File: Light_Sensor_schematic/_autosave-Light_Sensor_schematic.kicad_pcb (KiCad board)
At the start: 2 copper layers, 50 x 50 mm, 21 parts, among them IC1 TSL237S-LF, J1 Conn_01x03, J3 Conn_01x04_Male, U1 STM32L432KCUx, U2 STDC14, U3 TG-3541CE

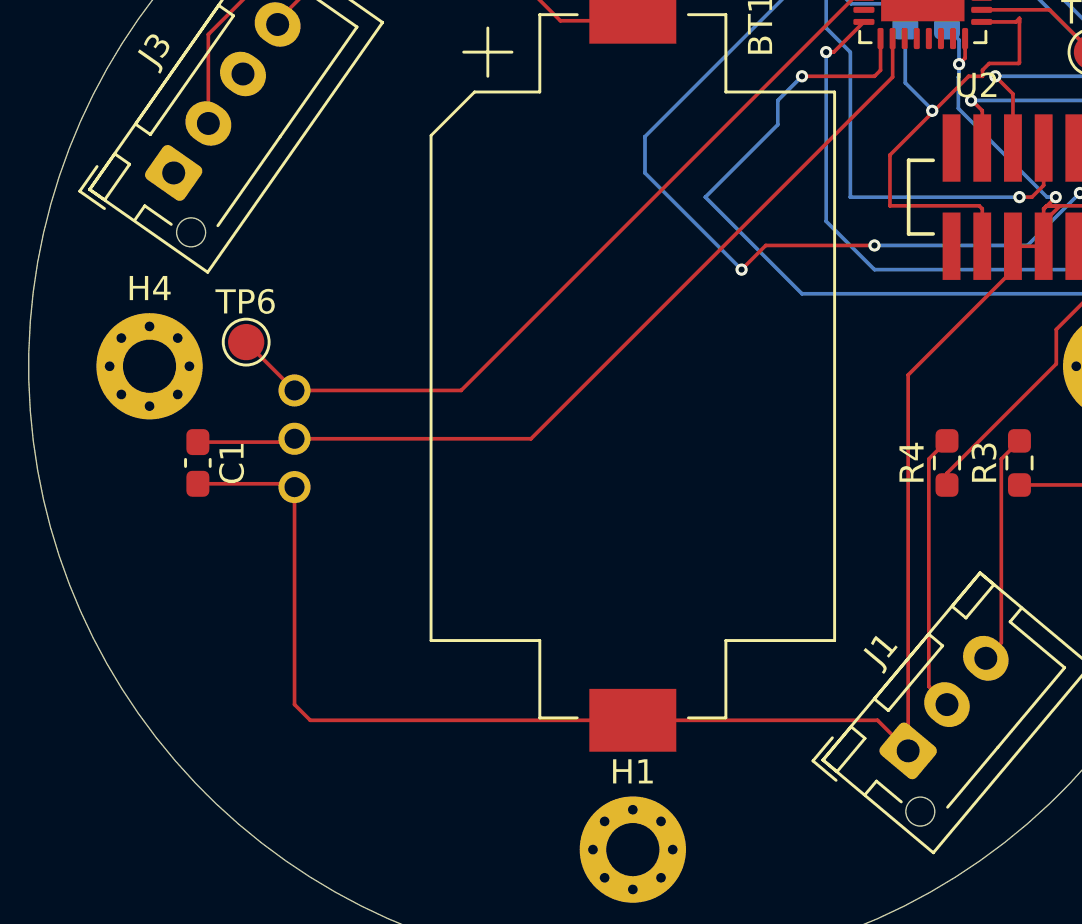
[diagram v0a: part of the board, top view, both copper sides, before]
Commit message: Lab 8
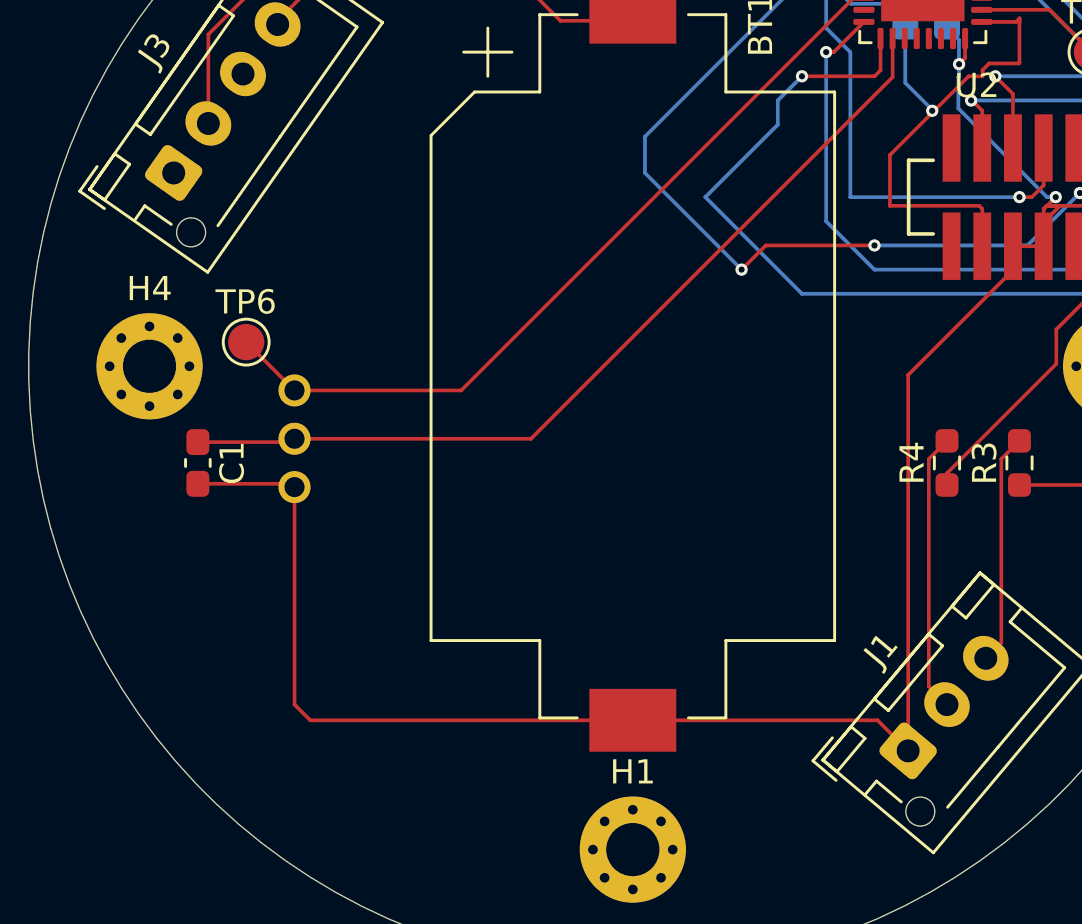
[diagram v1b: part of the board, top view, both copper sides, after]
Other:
- rule pad_to_mask_clearance: 0 -> 0.0508
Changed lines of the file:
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@@
     (pad_size 1.524 1.524)
     (pad_drill 0.762)
-    (pad_to_mask_clearance 0)
+    (pad_to_mask_clearance 0.0508)
     (aux_axis_origin 0 0)
     (visible_elements FFFFFF7F)
@@
       (outputformat 1)
       (mirror false)
-      (drillshape 1)
+      (drillshape 0)
       (scaleselection 1)
       (outputdirectory ""))
@@
       (effects (font (size 1 1) (thickness 0.15)))
     )
-    (pad 1 thru_hole roundrect (at 0 0 50) (size 1.7 1.95) (drill 0.95) (layers *.Cu *.Mask) (roundrect_rratio 0.147059)
+    (pad 1 thru_hole roundrect (at 0 0 50) (size 1.7 1.95) (drill 0.95) (layers *.Cu *.Mask) (roundrect_rratio 0.1470588235294118)
       (net 1 GND))
     (pad 2 thru_hole oval (at 2.5 0 50) (size 1.7 1.95) (drill 0.95) (layers *.Cu *.Mask)
@@
       (effects (font (size 1 1) (thickness 0.15)))
     )
-    (pad 1 thru_hole roundrect (at 0 0 55) (size 1.7 1.95) (drill 0.95) (layers *.Cu *.Mask) (roundrect_rratio 0.147059)
+    (pad 1 thru_hole roundrect (at 0 0 55) (size 1.7 1.95) (drill 0.95) (layers *.Cu *.Mask) (roundrect_rratio 0.1470588235294118)
       (net 8 "Net-(J3-Pad1)"))
     (pad 2 thru_hole oval (at 2.5 0 55) (size 1.7 1.95) (drill 0.95) (layers *.Cu *.Mask)
